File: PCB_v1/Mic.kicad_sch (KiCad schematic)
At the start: 10 parts, among them IC1 MIC_I2S_SPH0645, IC2 MIC_I2S_SPH0645

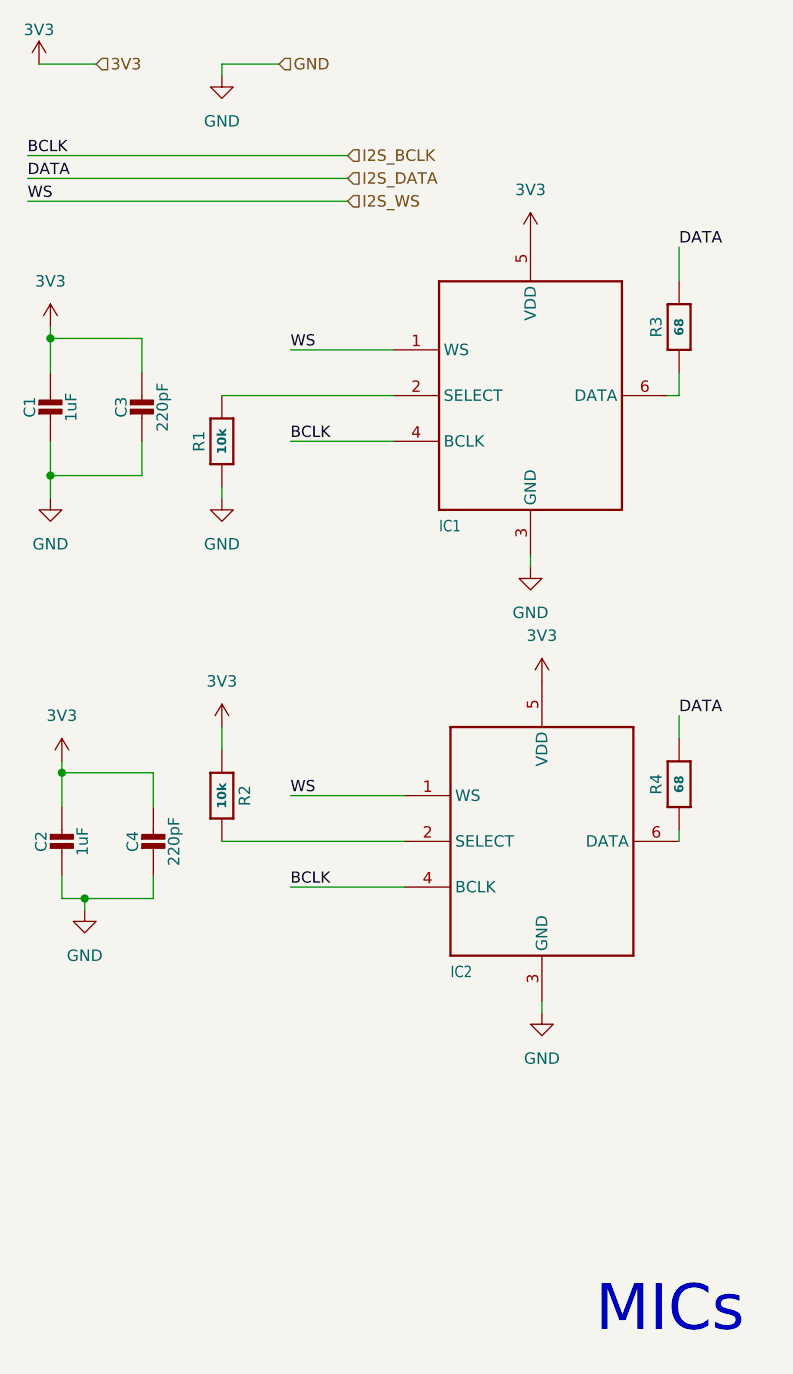
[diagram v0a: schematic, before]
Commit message: PCB updates
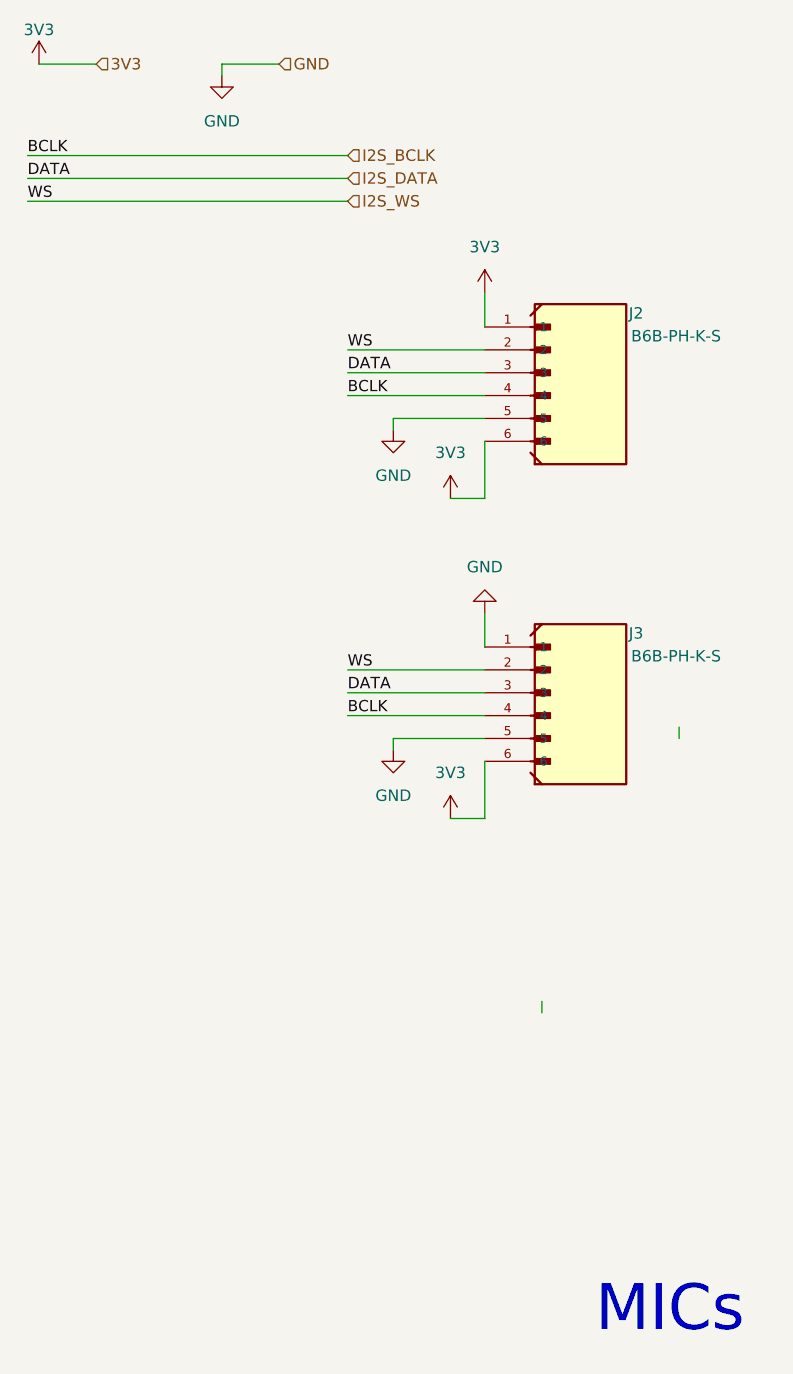
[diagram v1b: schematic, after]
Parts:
- removed C1, C2: 1uF, Capacitor_SMD:C_0805_2012Metric, symbol Adafruit I2S Mic SPK0415HM4H-eagle-import:CAP_CERAMIC0805-NOOUTLINE
- removed C3, C4: 220pF, Capacitor_SMD:C_0805_2012Metric, symbol Adafruit I2S Mic SPK0415HM4H-eagle-import:CAP_CERAMIC0805-NOOUTLINE
- removed IC1, IC2: MIC_I2S_SPH0645, SPH0645LM4H, symbol Adafruit I2S Mic SPK0415HM4H-eagle-import:MIC_I2S_SPH0645
- removed R1, R2: 10k, Resistor_SMD:R_0805_2012Metric, symbol Adafruit I2S Mic SPK0415HM4H-eagle-import:RESISTOR_0603_NOOUT
- removed R3, R4: 68, Resistor_SMD:R_0805_2012Metric, symbol Adafruit I2S Mic SPK0415HM4H-eagle-import:RESISTOR_0603_NOOUT
- added J2, J3: B6B-PH-K-S, GT_library:JST_B6B-PH-K-S, symbol GT_LIbrary:B6B-PH-K-S
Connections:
- net 3V3: now also J2.1, J2.6, J3.6
- net GND: now also J2.5, J3.1, J3.5
- net I2S_BCLK: now also J2.4, J3.4
- net I2S_DATA: now also J2.3, J3.3
- net I2S_WS: now also J2.2, J3.2
